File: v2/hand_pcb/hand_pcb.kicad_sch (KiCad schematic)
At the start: 56 parts, among them J1 Screw_Terminal_01x10, J10 8P8C, J2 Conn_01x08, J3 Conn_01x08, J4 Conn_01x02, J5 Conn_01x02, J9 Conn_02x02_Top_Bottom, M1 Motor_Servo_FB, M10 Motor_Servo_FB, M2 Motor_Servo_FB, M3 Motor_Servo_FB, M4 Motor_Servo_FB, M5 Motor_Servo_FB, M6 Motor_Servo_FB, M7 Motor_Servo_FB, M8 Motor_Servo_FB, M9 Motor_Servo_FB, Q1 Q_NMOS_GDS, Q2 Q_NMOS_GDS, Q3 Q_NMOS_GDS, Q4 Q_NMOS_GDS, Q5 Q_NMOS_GDS, U1 PCA9685PW, U2 MCP23017_SP

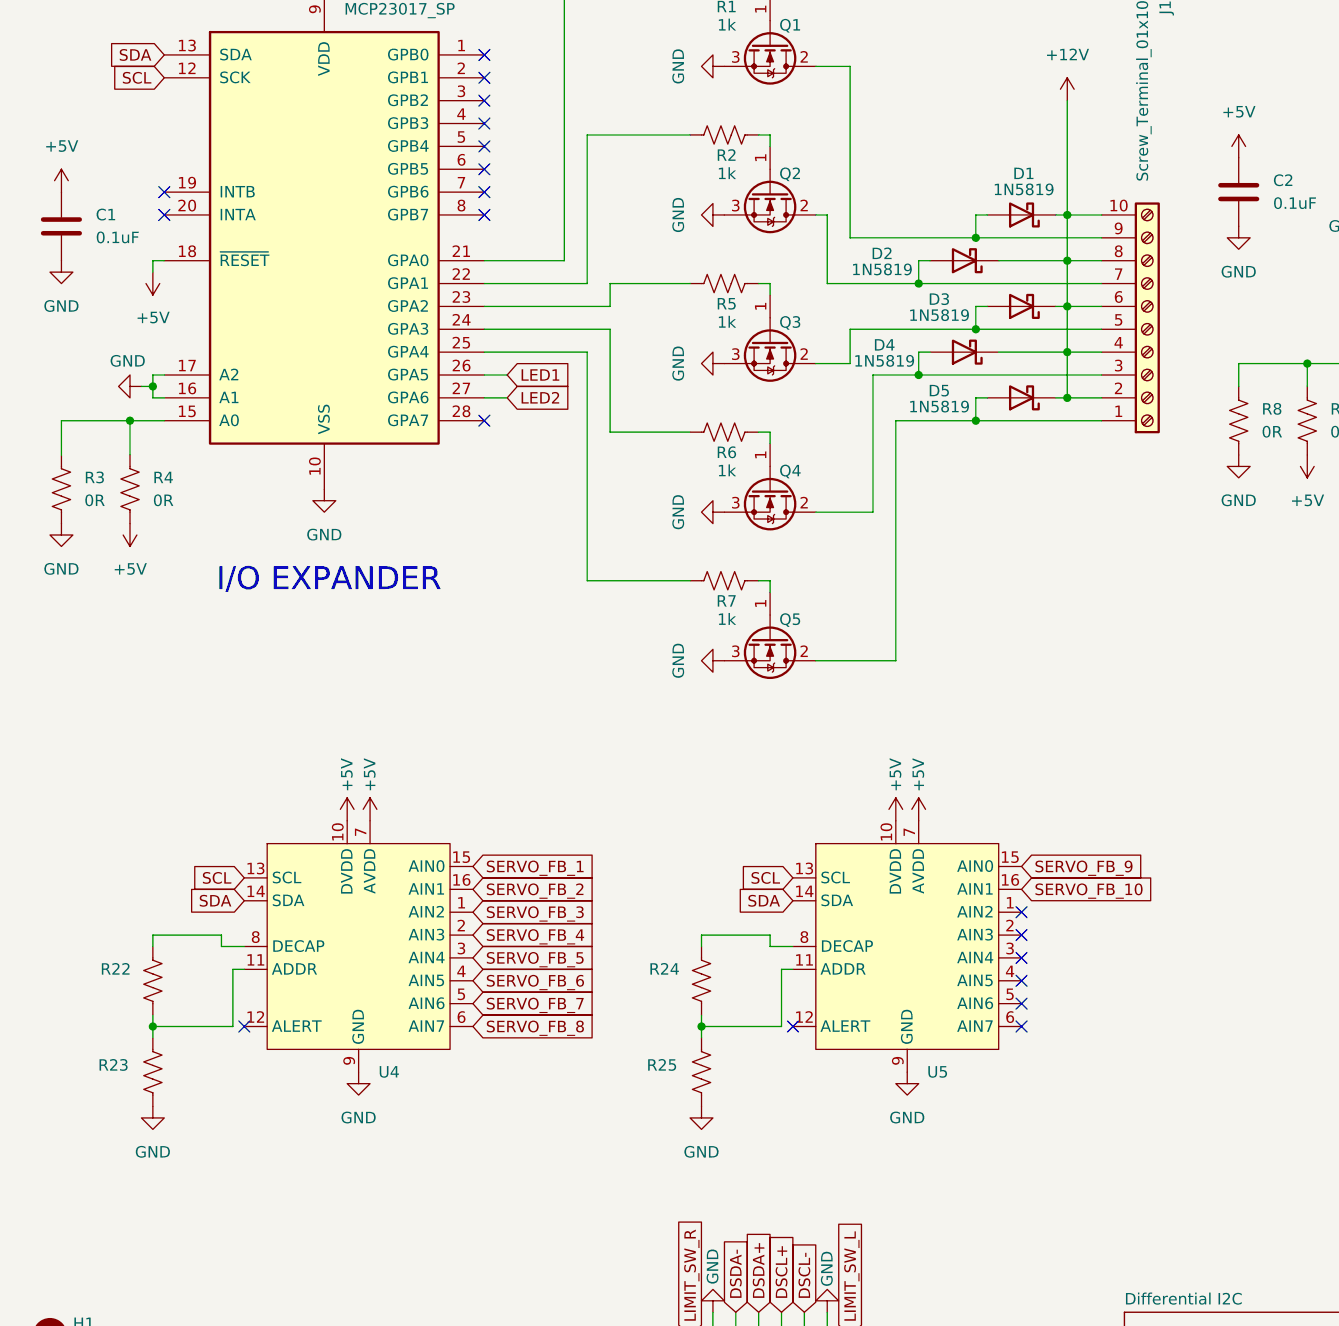
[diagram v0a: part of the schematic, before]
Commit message: Doing some things
Crossing some ts and dotting some is. Making v3 of the BOM.
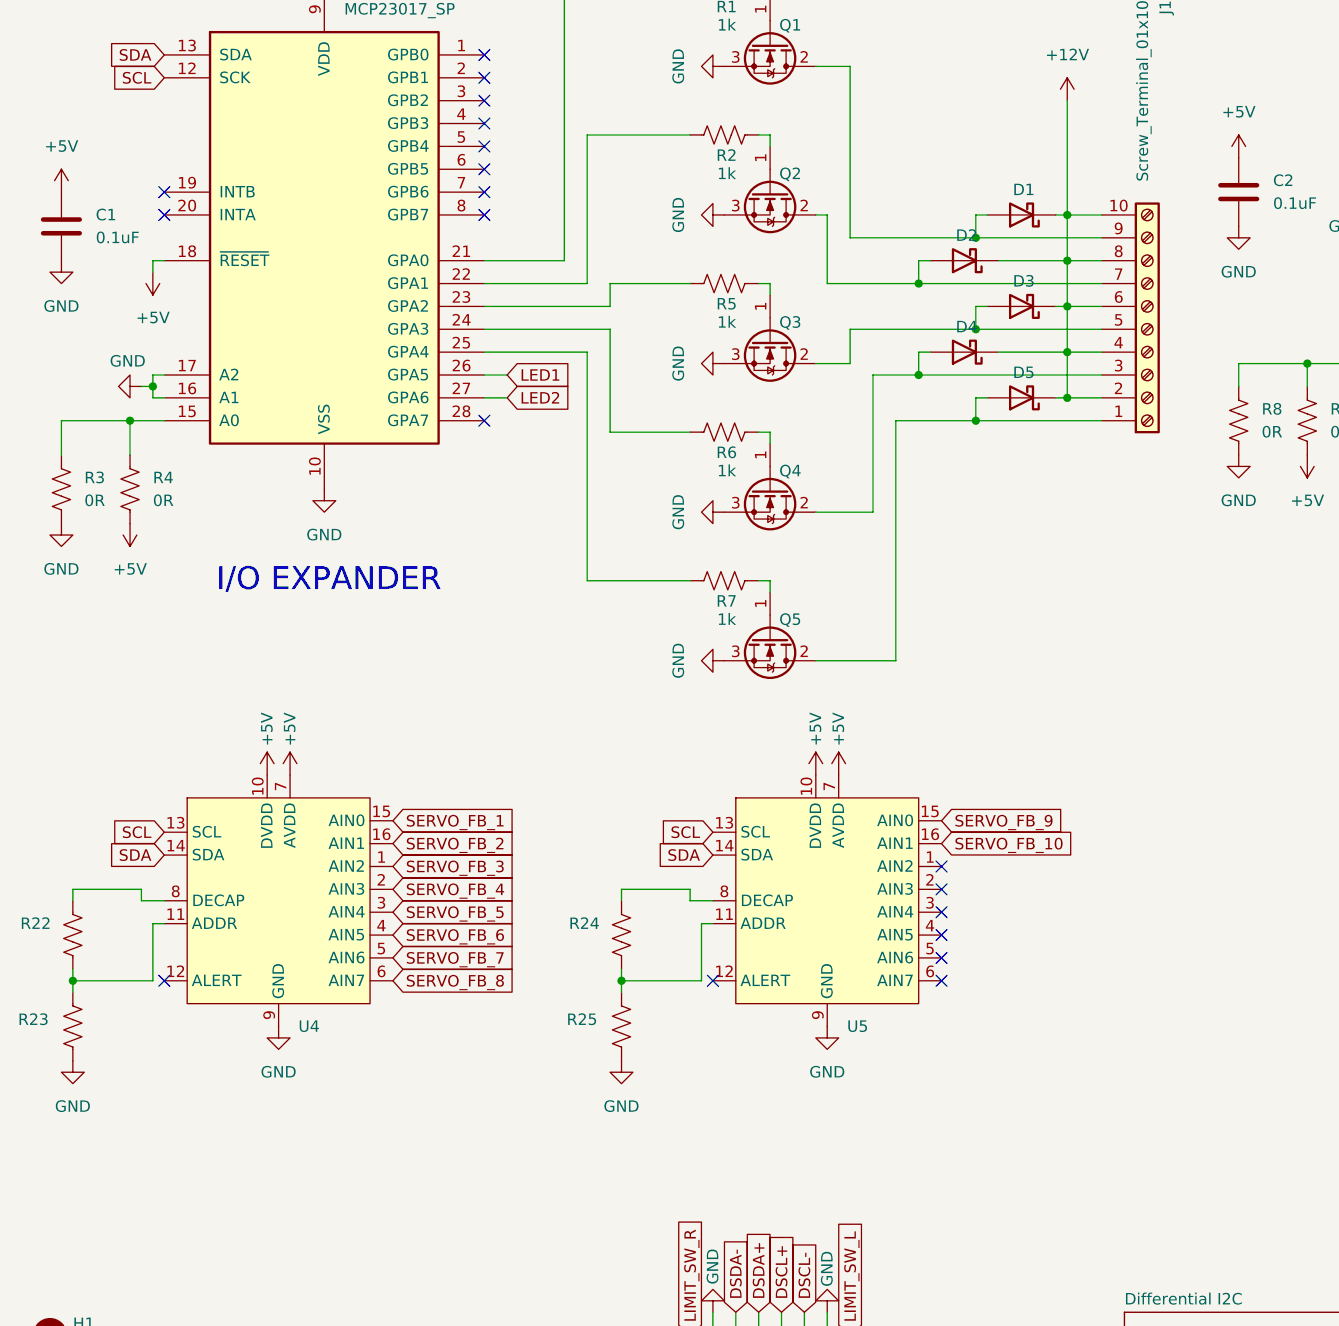
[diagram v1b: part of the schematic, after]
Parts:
- D1, D2, D3, D4, D5: value 1N5819 -> SB5100-T; footprint Diode_THT:D_DO-41_SOD81_P10.16mm_Horizontal -> Diode_THT:D_DO-201AD_P12.70mm_Horizontal; Digikey (none) -> https://www.digikey.ca/en/products/detail/diodes-incorporat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
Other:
- moved on the sheet: R22, R23, R24, R25, U4, U5

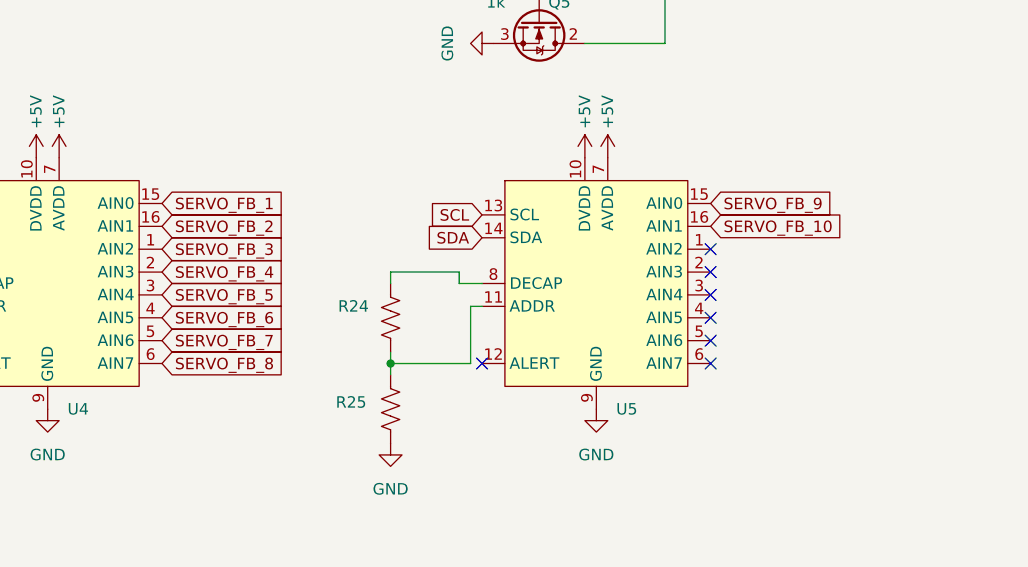
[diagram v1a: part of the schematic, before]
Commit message: Doing some things
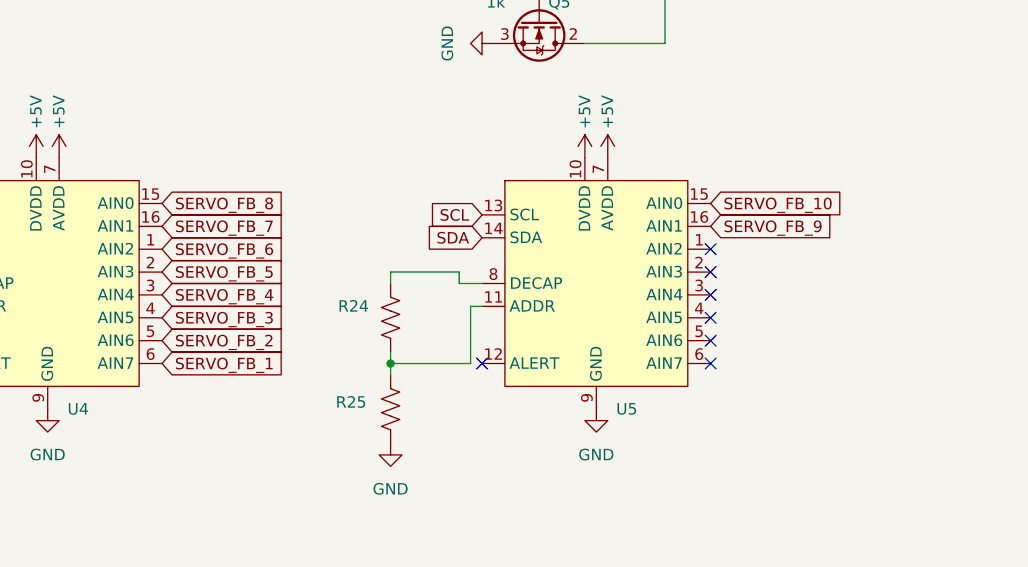
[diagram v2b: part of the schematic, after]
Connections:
- net SERVO_FB_1: now also U4.6 (AIN7); no longer U4.15 (AIN0)
- net SERVO_FB_10: now also U5.15 (AIN0); no longer U5.16 (AIN1)
- net SERVO_FB_2: now also U4.5 (AIN6); no longer U4.16 (AIN1)
- net SERVO_FB_3: now also U4.4 (AIN5); no longer U4.1 (AIN2)
- net SERVO_FB_4: now also U4.3 (AIN4); no longer U4.2 (AIN3)
- net SERVO_FB_5: now also U4.2 (AIN3); no longer U4.3 (AIN4)
- net SERVO_FB_6: now also U4.1 (AIN2); no longer U4.4 (AIN5)
- net SERVO_FB_7: now also U4.16 (AIN1); no longer U4.5 (AIN6)
- net SERVO_FB_8: now also U4.15 (AIN0); no longer U4.6 (AIN7)
- net SERVO_FB_9: now also U5.16 (AIN1); no longer U5.15 (AIN0)
